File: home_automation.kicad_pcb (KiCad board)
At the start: 2 copper layers, 48 parts, among them J1 AC_in, J2 NodeMCU Header, J3 NodeMCU Header, J4 Sw_1, J5 DHT11, J6 Sw_2, J7 Sw_3, J8 Sw_4, K1 Relay_SPDT, K2 Relay_SPDT, K3 Relay_SPDT, K4 Relay_SPDT, Q1 D882, Q2 D882, Q3 D882, Q4 D882, SW1 SW_DIP_x02, SW2 SW_DIP_x02, SW3 SW_DIP_x02, SW4 SW_DIP_x02, U1 PC817, U2 PC817, U3 LM7805_TO220, U4 PC817, U5 PC817, U6 NodeMCU

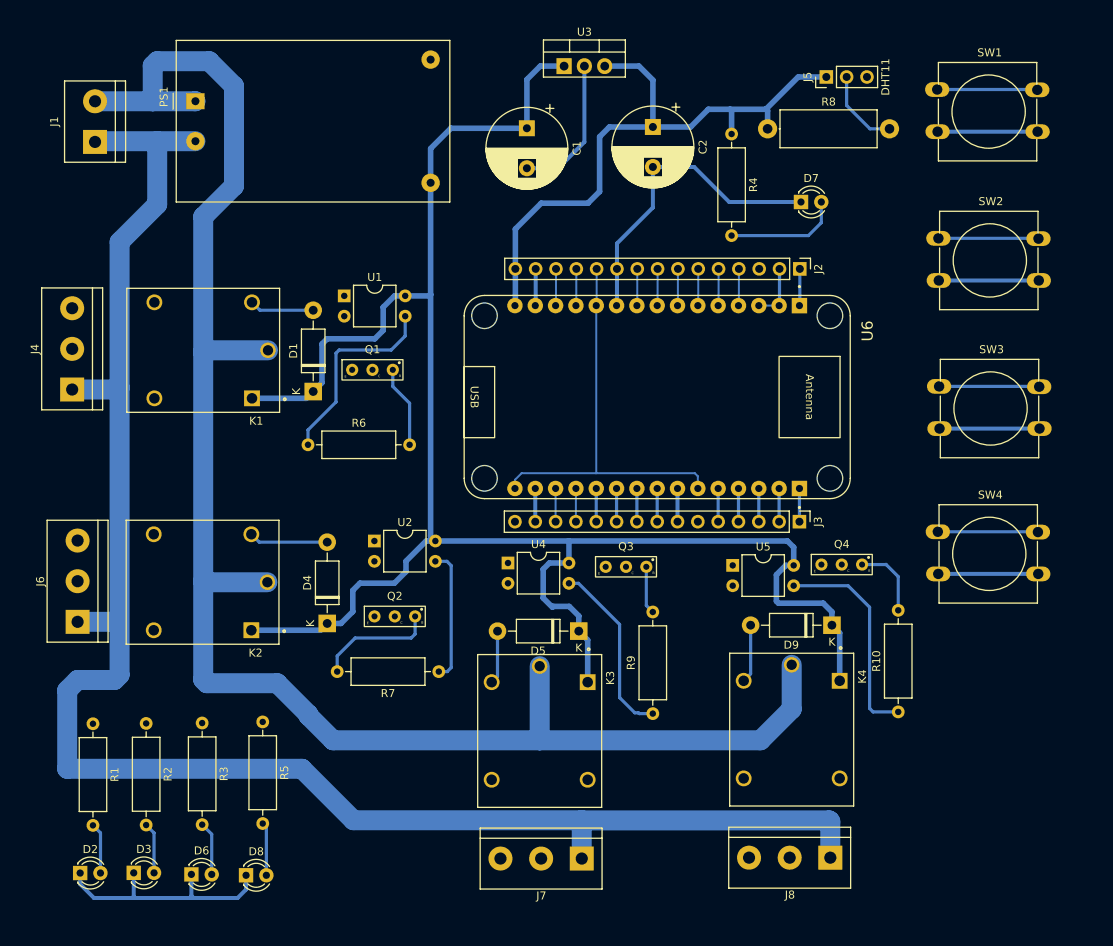
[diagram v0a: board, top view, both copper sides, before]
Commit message: Routing Completed
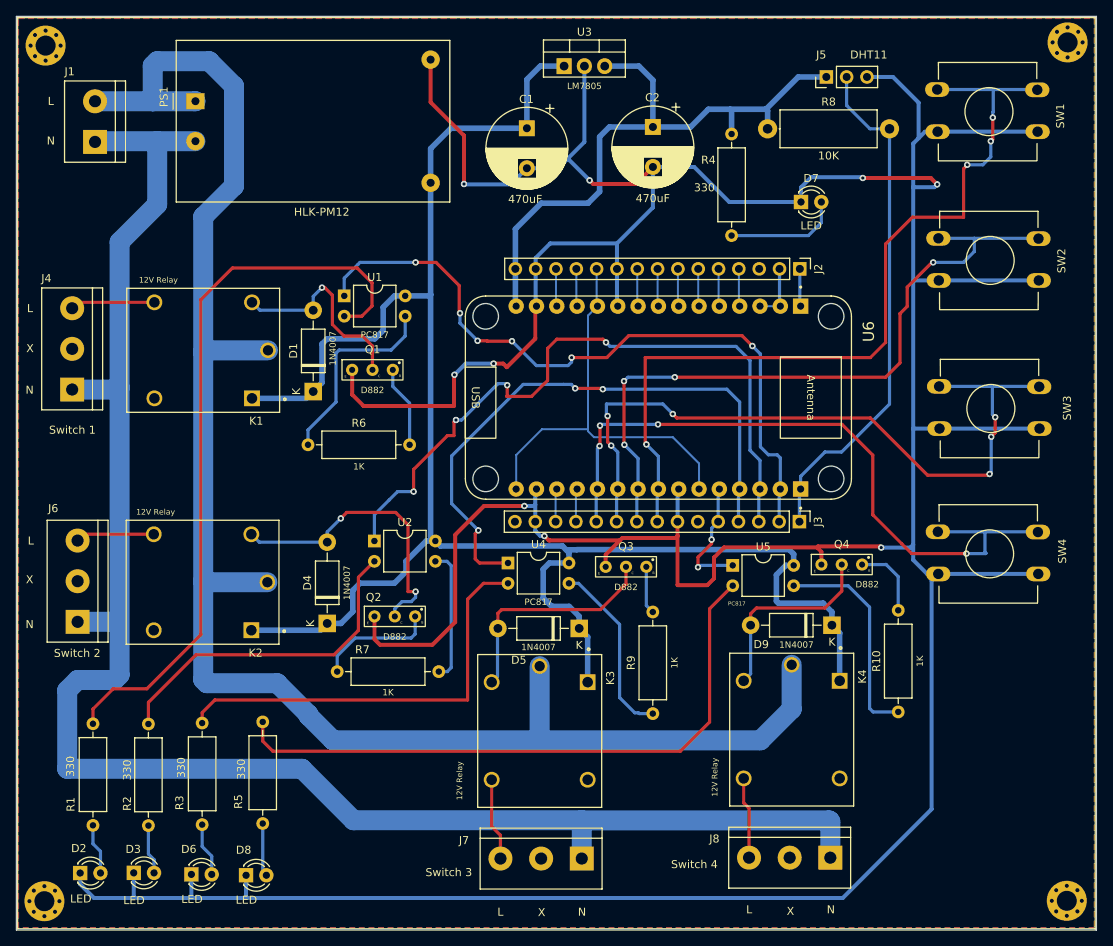
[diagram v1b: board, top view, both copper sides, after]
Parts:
- added REF**: MountingHole_2.5mm_Pad_Via, MountingHole:MountingHole_2.5mm_Pad_Via, F.Cu at (211.2, 43.2)
- added REF**: MountingHole_2.5mm_Pad_Via, MountingHole:MountingHole_2.5mm_Pad_Via, F.Cu at (83.5, 43.6)
- added REF**: MountingHole_2.5mm_Pad_Via, MountingHole:MountingHole_2.5mm_Pad_Via, F.Cu at (211.1, 150.6)
- added REF**: MountingHole_2.5mm_Pad_Via, MountingHole:MountingHole_2.5mm_Pad_Via, F.Cu at (83.3, 150.6)
- added REF**: ESD-Logo_8.9x8mm_SilkScreen, Symbol:ESD-Logo_8.9x8mm_SilkScreen, B.Cu at (97.0, 52.6)
- added REF**: KiCad-Logo2_6mm_SilkScreen, Symbol:KiCad-Logo2_6mm_SilkScreen, B.Cu at (199.9, 130.7)
- added REF**: OSHW-Logo2_14.6x12mm_SilkScreen, Symbol:OSHW-Logo2_14.6x12mm_SilkScreen, B.Cu at (96.3, 134.9)
- K1, K2, K3, K4: value Relay_SPDT -> 12V Relay
- U3: value LM7805_TO220 -> LM7805
- moved D5 0.34 mm to (150.2, 116.5)
- moved R2 0.29 mm to (96.3, 128.4)
- moved U6 0.17 mm to (160.1, 87.7)
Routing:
- net GND: track 151.8 -> 566.4 mm, vias 0 -> 9
- net Net-(R1-Pad1): track 0.00 -> 91.8 mm
- net /D5: track 16.7 -> 106.7 mm, vias 0 -> 4
- net /D1: track 4.15 -> 88.7 mm, vias 0 -> 6
- net /D2: track 4.15 -> 88.3 mm, vias 0 -> 4
- net Net-(R5-Pad1): track 0.00 -> 78.5 mm
- net /D7: track 16.7 -> 90.9 mm, vias 0 -> 6
- net /D6: track 16.7 -> 88.1 mm, vias 0 -> 4
- net /D3: track 4.15 -> 74.4 mm, vias 0 -> 3
- net /D8: track 16.7 -> 86.9 mm, vias 0 -> 4
- net Net-(R3-Pad1): track 0.00 -> 53.6 mm
- net /D0: track 14.3 -> 65.1 mm
- net Net-(R2-Pad1): track 0.00 -> 42.1 mm
- net /Collector_2: track 9.89 -> 37.1 mm, vias 0 -> 2
- net /Collector_3: track 6.68 -> 28.6 mm
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- added copper zone on B.Cu, net /3V3-1
- added copper zone on F.Cu, net GND
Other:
- board outline added: 135 x 114.2 mm
- board text added: "Home Automation And Temperature Sensor"
- board text added: "L"
- board text added: "N"
- board text added: "Switch 1"
- board text added: "Switch 2"
- board text added: "Switch 3"
- board text added: "Switch 4"
- board text added: "X"
